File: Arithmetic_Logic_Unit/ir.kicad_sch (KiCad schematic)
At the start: 19 parts, among them IC1 SN54173J, IC2 SN54173J, U1 74LS245

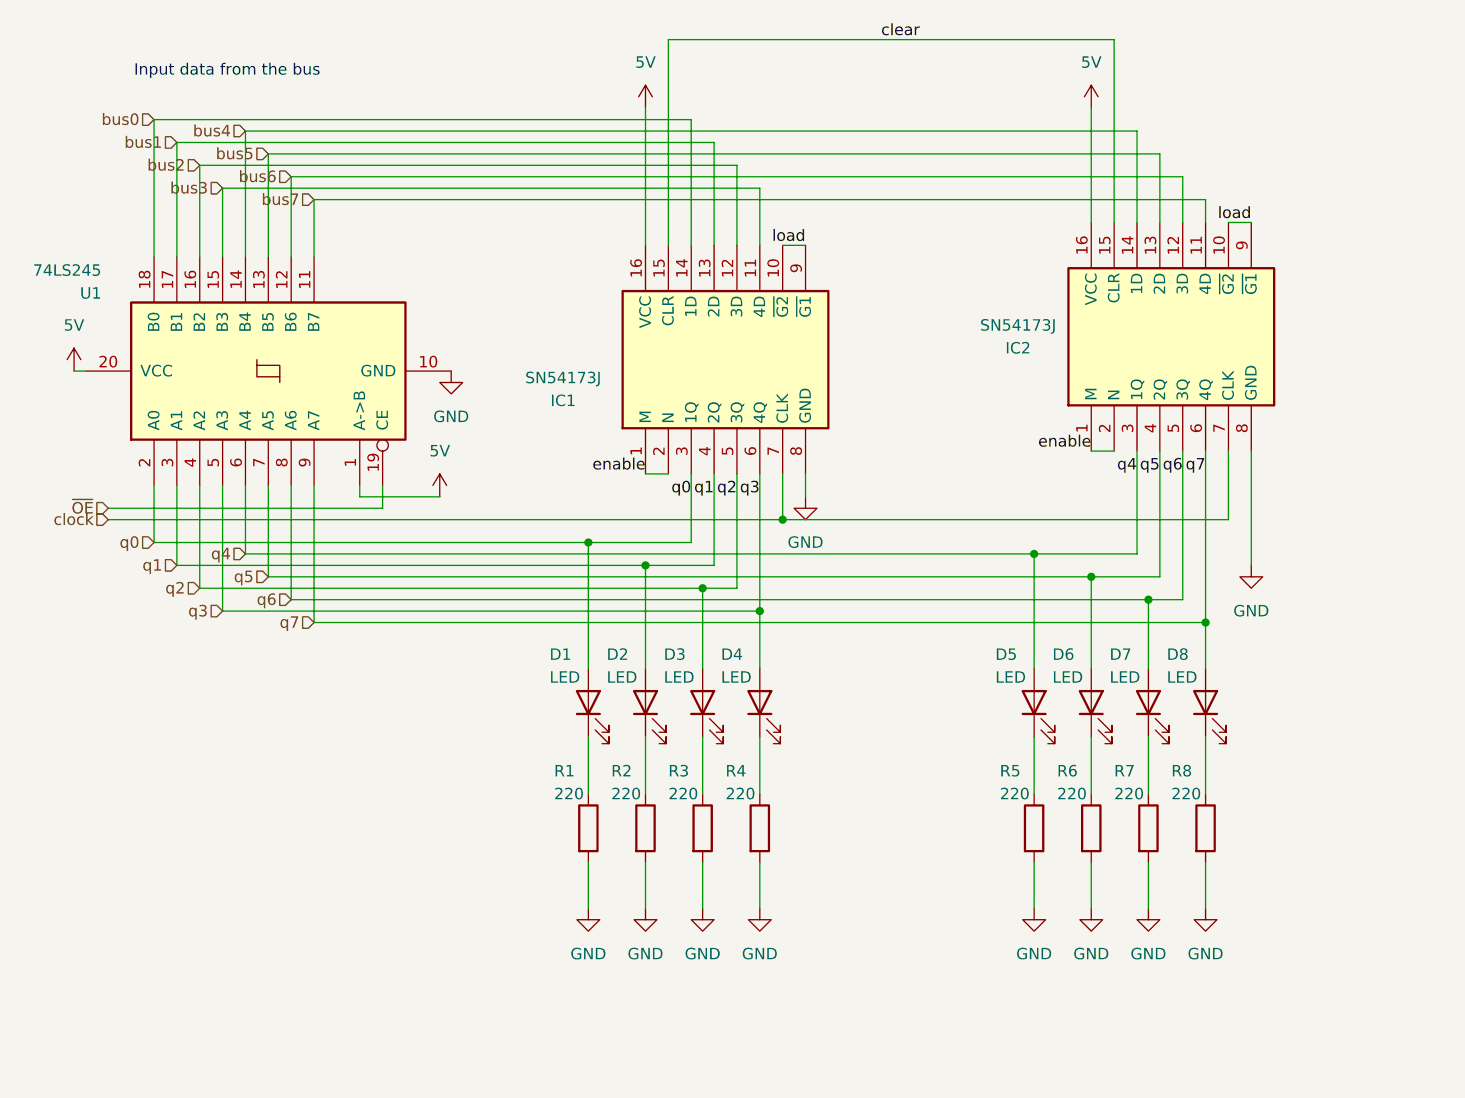
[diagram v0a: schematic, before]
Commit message: added instructional register
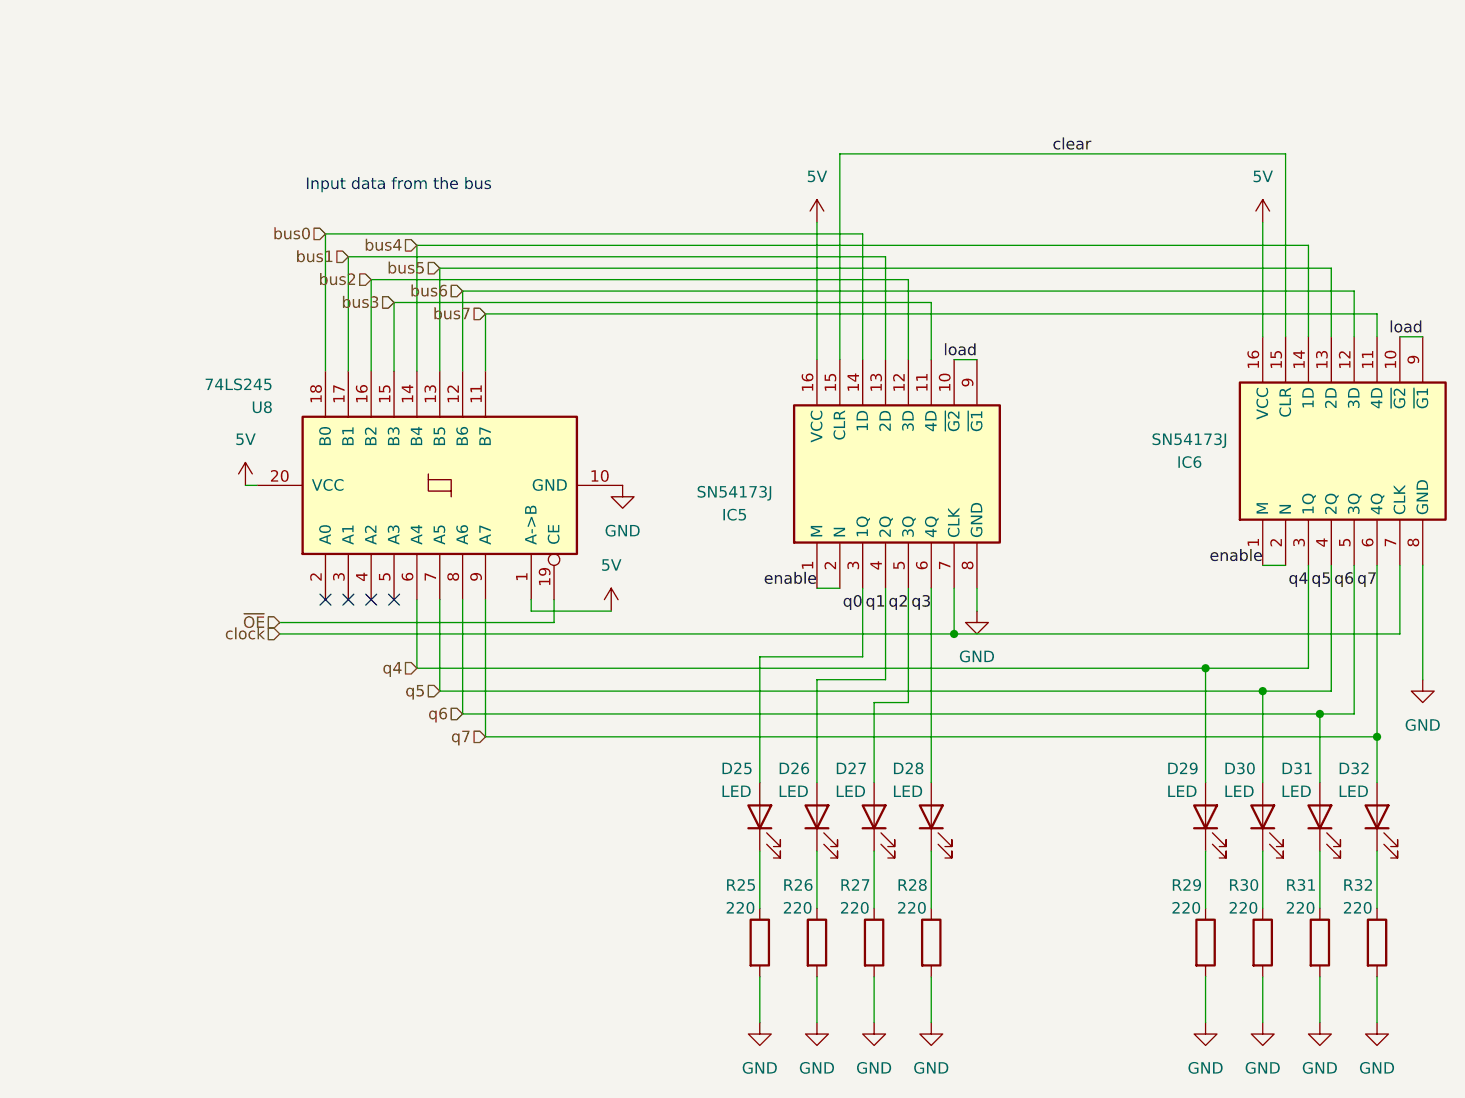
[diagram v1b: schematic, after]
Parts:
- removed D1, D2, D3, D4, D5, D6, D7, D8: LED, symbol Device:LED
- removed IC1, IC2: SN54173J, footprints:SN54173J, symbol SN54173J:SN54173J
- removed R1, R2, R3, R4, R5, R6, R7, R8: 220, symbol Device:R
- removed U1: 74LS245, symbol 74xx:74LS245
- added D25, D26, D27, D28, D29, D30, D31, D32: LED, symbol Device:LED
- added IC5, IC6: SN54173J, footprints:SN54173J, symbol SN54173J:SN54173J
- added R25, R26, R27, R28, R29, R30, R31, R32: 220, symbol Device:R
- added U8: 74LS245, symbol 74xx:74LS245
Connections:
- net 5V: now also IC5.16 (VCC), IC6.16 (VCC), U8.1 (A->B), U8.20 (VCC)
- net GND: now also IC5.8 (GND), IC6.8 (GND), R25.2, R26.2, R27.2, R28.2, R29.2, R30.2, R31.2, R32.2, U8.10 (GND)
- net bus0: now also IC5.14 (1D), U8.18 (B0)
- net bus1: now also IC5.13 (2D), U8.17 (B1)
- net bus2: now also IC5.12 (3D), U8.16 (B2)
- net bus3: now also IC5.11 (4D), U8.15 (B3)
- net bus4: now also IC6.14 (1D), U8.14 (B4)
- net bus5: now also IC6.13 (2D), U8.13 (B5)
- net bus6: now also IC6.12 (3D), U8.12 (B6)
- net bus7: now also IC6.11 (4D), U8.11 (B7)
- net clear: now also IC5.15 (CLR), IC6.15 (CLR)
- net clock: now also IC5.7 (CLK), IC6.7 (CLK)
- net enable: now also IC5.1 (M), IC5.2 (N), IC6.1 (M), IC6.2 (N)
- net load: now also IC5.10 (~{G2}), IC5.9 (~{G1}), IC6.10 (~{G2}), IC6.9 (~{G1})
- net q0: now also D25.2 (A), IC5.3 (1Q)
- net q1: now also D26.2 (A), IC5.4 (2Q)
- net q2: now also D27.2 (A), IC5.5 (3Q)
- net q3: now also D28.2 (A), IC5.6 (4Q)
- net q4: now also D29.2 (A), IC6.3 (1Q), U8.6 (A4)
- net q5: now also D30.2 (A), IC6.4 (2Q), U8.7 (A5)
- net q6: now also D31.2 (A), IC6.5 (3Q), U8.8 (A6)
- net q7: now also D32.2 (A), IC6.6 (4Q), U8.9 (A7)
- net ~{OE}: now also U8.19 (CE)
- new net: D29.1 (K), R29.1
- new net: D32.1 (K), R32.1
- new net: D30.1 (K), R30.1
- new net: D28.1 (K), R28.1
- new net: D27.1 (K), R27.1
- new net: D25.1 (K), R25.1
- new net: D26.1 (K), R26.1
- new net: D31.1 (K), R31.1
- no-connect marks 0 -> 4
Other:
- title: Registers -> (none)
